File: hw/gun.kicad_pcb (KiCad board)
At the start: 2 copper layers, 65 x 45 mm, 53 parts, among them J1 SWD_01X04, J2 IDC_02X05, SW1 FUSE, SW2 BANG, U1 OSRB38C9BA, U2 ULN2003, U3 ULN2003, U4 MCP1826S, U5 74AHC1G08, U6 STM32F042F6Px, U7 74AHC1G08, U8 MCP1826S, U9 74AHC1G08

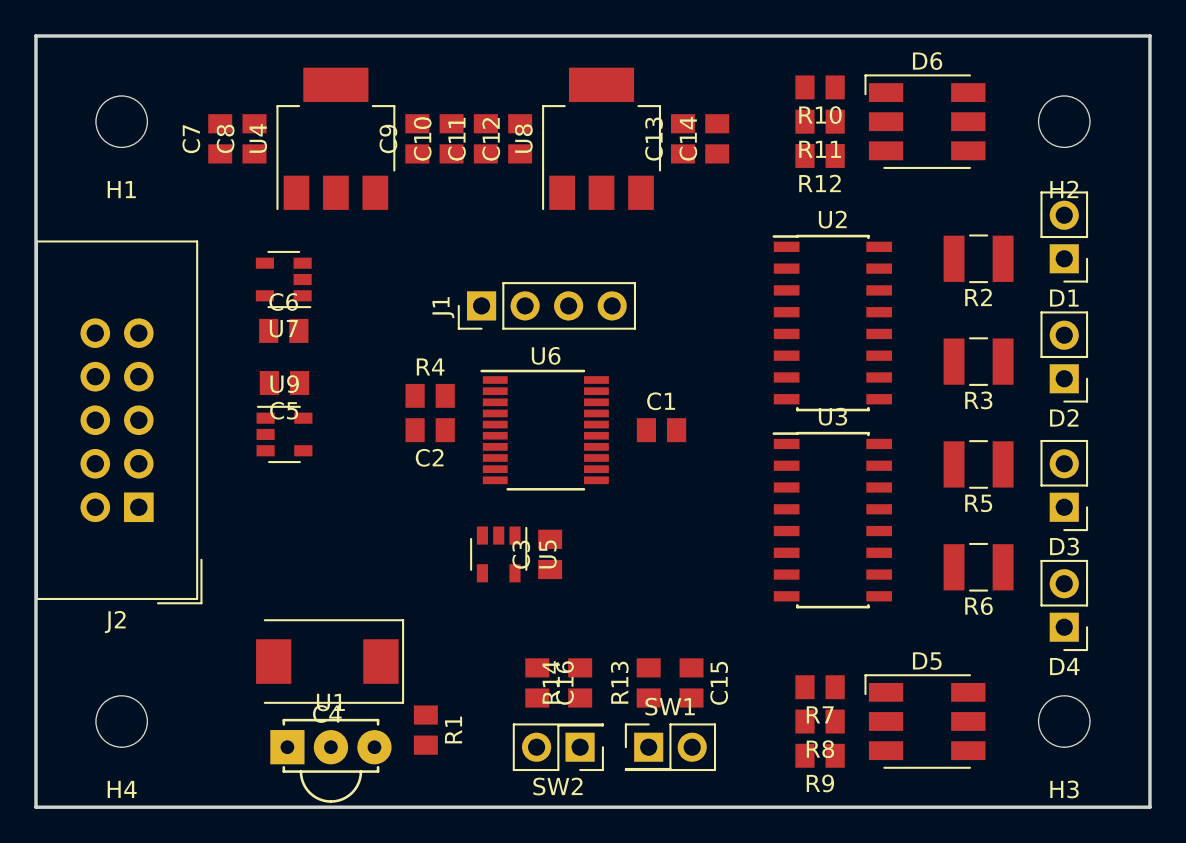
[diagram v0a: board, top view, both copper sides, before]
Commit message: updated pcb
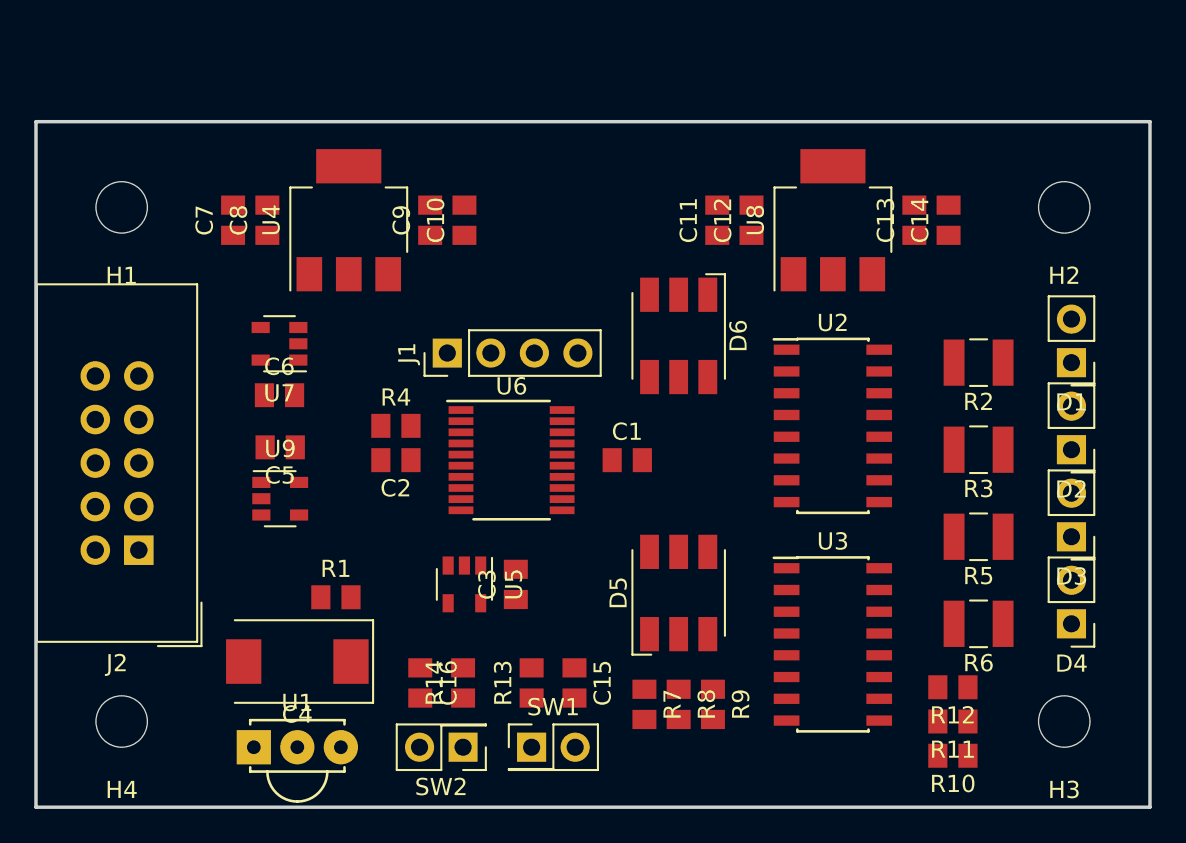
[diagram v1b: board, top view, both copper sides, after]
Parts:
- moved R10 39.8 mm to (178.5, 122.0)
- moved R11 35.8 mm to (178.5, 120.0)
- moved R12 32.0 mm to (178.5, 118.0)
- moved D6 19.1 mm to (162.5, 97.5), turned to 270 degrees
- moved D5 16.3 mm to (162.5, 112.5), turned to 90 degrees
- moved C11 14.3 mm to (164.8, 90.8)
- moved C12 14.3 mm to (166.8, 90.8)
- moved C13 14.3 mm to (176.2, 90.8)
- moved C14 14.3 mm to (178.2, 90.8)
- moved U8 14.3 mm to (171.5, 90.8)
- moved R7 10.3 mm to (160.5, 119.0), turned to 270 degrees
- moved R1 9.36 mm to (142.5, 112.8), turned to 0 degrees
- moved R8 8.31 mm to (162.5, 119.0), turned to 270 degrees
- moved U3 7.25 mm to (171.5, 115.5)
- moved R9 6.93 mm to (164.5, 119.0), turned to 270 degrees
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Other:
- board size 65 x 45 mm -> 65 x 40 mm
